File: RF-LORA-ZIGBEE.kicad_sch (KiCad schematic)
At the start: 2 parts, among them J4 xAnt, U6 Ai-Thinker-Ra-02

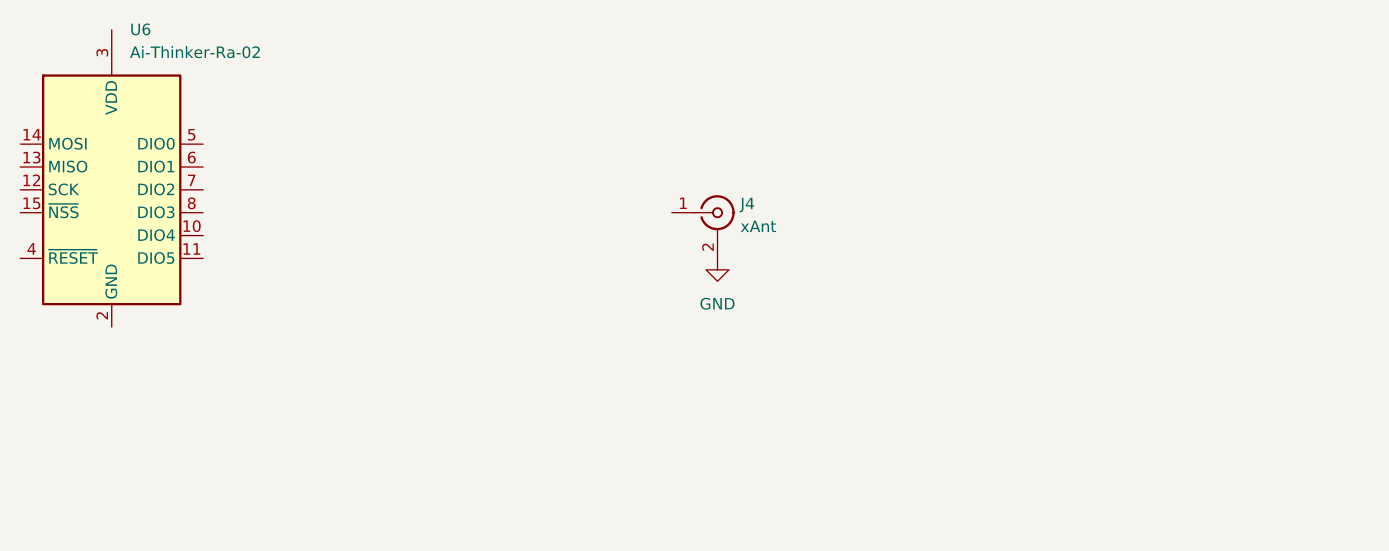
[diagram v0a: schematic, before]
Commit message: Add RS485 Layout.
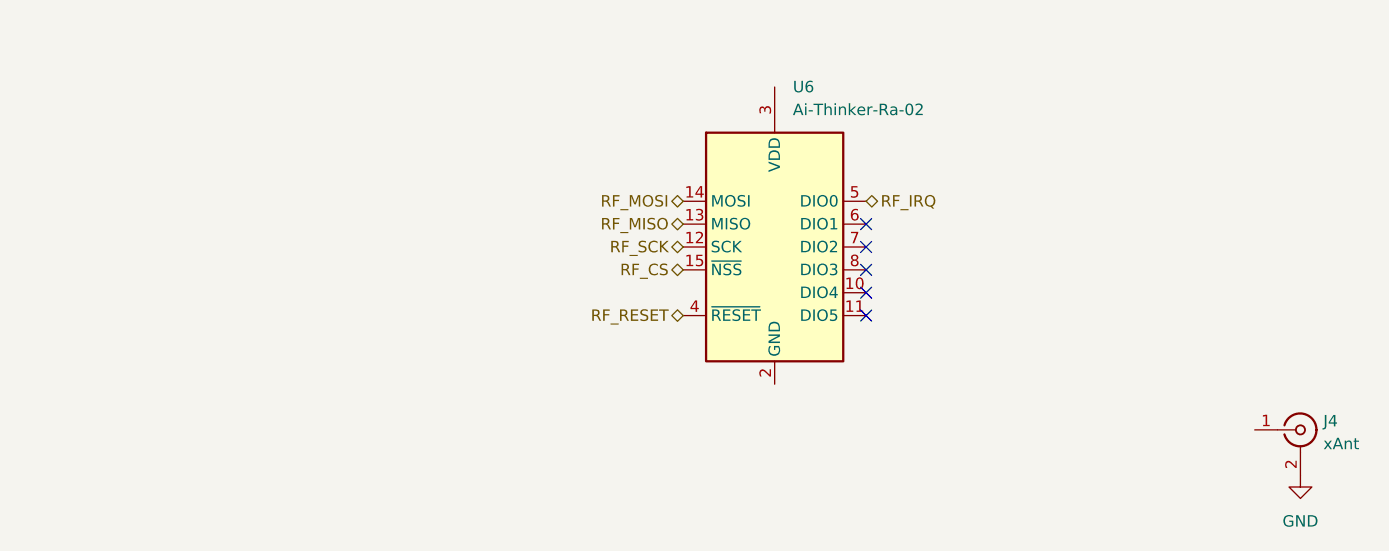
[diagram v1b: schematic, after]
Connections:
- net RF_SCK: now reaches U6.12 (SCK)
- net RF_MISO: now reaches U6.13 (MISO)
- net RF_MOSI: now reaches U6.14 (MOSI)
- net RF_CS: now reaches U6.15 (~{NSS})
- net RF_RESET: now reaches U6.4 (~{RESET})
- net RF_IRQ: now reaches U6.5 (DIO0)
- no-connect marks 0 -> 5
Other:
- moved on the sheet: J4, U6
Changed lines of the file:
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@@
 (kicad_sch (version 20211123) (generator eeschema)
   (paper "A4")
-  (symbol (lib_id "RF_Module:Ai-Thinker-Ra-02") (at 138.43 90.17 0) (unit 1)
+  (no_connect (at 222.25 104.14))
+  (no_connect (at 222.25 101.6))
+  (no_connect (at 222.25 93.98))
+  (no_connect (at 222.25 96.52))
+  (no_connect (at 222.25 99.06))
+  (hierarchical_label "RF_IRQ" (shape bidirectional) (at 222.25 91.44 0)
+    (effects (font (size 1.27 1.27)) (justify left))
+  )
+  (hierarchical_label "RF_CS" (shape bidirectional) (at 201.93 99.06 180)
+    (effects (font (size 1.27 1.27)) (justify right))
+  )
+  (hierarchical_label "RF_SCK" (shape bidirectional) (at 201.93 96.52 180)
+    (effects (font (size 1.27 1.27)) (justify right))
+  )
+  (hierarchical_label "RF_MOSI" (shape bidirectional) (at 201.93 91.44 180)
+    (effects (font (size 1.27 1.27)) (justify right))
+  )
+  (hierarchical_label "RF_RESET" (shape bidirectional) (at 201.93 104.14 180)
+    (effects (font (size 1.27 1.27)) (justify right))
+  )
+  (hierarchical_label "RF_MISO" (shape bidirectional) (at 201.93 93.98 180)
+    (effects (font (size 1.27 1.27)) (justify right))
+  )
+  (symbol (lib_id "RF_Module:Ai-Thinker-Ra-02") (at 212.09 96.52 0) (unit 1)
     (in_bom yes) (on_board yes) (fields_autoplaced)
-    (property "Reference" "U6" (id 0) (at 140.4494 72.39 0)
+    (property "Reference" "U6" (id 0) (at 214.1094 78.74 0)
       (effects (font (size 1.27 1.27)) (justify left))
     )
-    (property "Value" "Ai-Thinker-Ra-02" (id 1) (at 140.4494 74.93 0)
+    (property "Value" "Ai-Thinker-Ra-02" (id 1) (at 214.1094 81.28 0)
       (effects (font (size 1.27 1.27)) (justify left))
     )
-    (property "Footprint" "RF_Module:Ai-Thinker-Ra-01-LoRa" (id 2) (at 163.83 100.33 0)
+    (property "Footprint" "RF_Module:Ai-Thinker-Ra-01-LoRa" (id 2) (at 237.49 106.68 0)
       (effects (font (size 1.27 1.27)) hide)
     )
-    (property "Datasheet" "http://wiki.ai-thinker.com/_media/lora/docs/c048ps01a1_ra-02_product_specification_v1.1.pdf" (id 3) (at 140.97 71.12 0)
+    (property "Datasheet" "http://wiki.ai-thinker.com/_media/lora/docs/c048ps01a1_ra-02_product_specification_v1.1.pdf" (id 3) (at 214.63 77.47 0)
       (effects (font (size 1.27 1.27)) hide)
     )
@@
     (pin "9")
   )
-  (symbol (lib_id "power:GND") (at 205.74 97.79 0) (unit 1)
+  (symbol (lib_id "power:GND") (at 270.51 121.92 0) (unit 1)
     (in_bom yes) (on_board yes) (fields_autoplaced)
-    (property "Reference" "#PWR0162" (id 0) (at 205.74 104.14 0)
+    (property "Reference" "#PWR0162" (id 0) (at 270.51 128.27 0)
       (effects (font (size 1.27 1.27)) hide)
     )
-    (property "Value" "GND" (id 1) (at 205.74 102.87 0))
-    (property "Footprint" "" (id 2) (at 205.74 97.79 0)
+    (property "Value" "GND" (id 1) (at 270.51 127 0))
+    (property "Footprint" "" (id 2) (at 270.51 121.92 0)
       (effects (font (size 1.27 1.27)) hide)
     )
-    (property "Datasheet" "" (id 3) (at 205.74 97.79 0)
+    (property "Datasheet" "" (id 3) (at 270.51 121.92 0)
       (effects (font (size 1.27 1.27)) hide)
     )
     (pin "1")
   )
-  (symbol (lib_id "Connector:Conn_Coaxial") (at 205.74 92.71 0) (unit 1)
+  (symbol (lib_id "Connector:Conn_Coaxial") (at 270.51 116.84 0) (unit 1)
     (in_bom yes) (on_board yes) (fields_autoplaced)
-    (property "Reference" "J4" (id 0) (at 208.28 91.7331 0)
+    (property "Reference" "J4" (id 0) (at 273.05 115.8631 0)
       (effects (font (size 1.27 1.27)) (justify left))
     )
-    (property "Value" "xAnt" (id 1) (at 208.28 94.2731 0)
+    (property "Value" "xAnt" (id 1) (at 273.05 118.4031 0)
       (effects (font (size 1.27 1.27)) (justify left))
     )
-    (property "Footprint" "Anh_Footprints:Connector_Coaxial_SMA" (id 2) (at 205.74 92.71 0)
+    (property "Footprint" "Anh_Footprints:Connector_Coaxial_SMA" (id 2) (at 270.51 116.84 0)
       (effects (font (size 1.27 1.27)) hide)
     )
-    (property "Datasheet" " ~" (id 3) (at 205.74 92.71 0)
+    (property "Datasheet" " ~" (id 3) (at 270.51 116.84 0)
       (effects (font (size 1.27 1.27)) hide)
     )
